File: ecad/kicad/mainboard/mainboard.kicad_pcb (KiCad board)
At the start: 2 copper layers, 99.1 x 81.3 mm, 37 parts, among them IC1 74HC86, J1 SENSORS, J2 CONN_06SILK_FEMALE_PTH, J3 CONN_06SILK_FEMALE_PTH, J4 POWER, J5 SERIAL, M1 Left Motor, M2 Right Motor, U1 Arduino_Nano, U2 TB6612FNG-Module

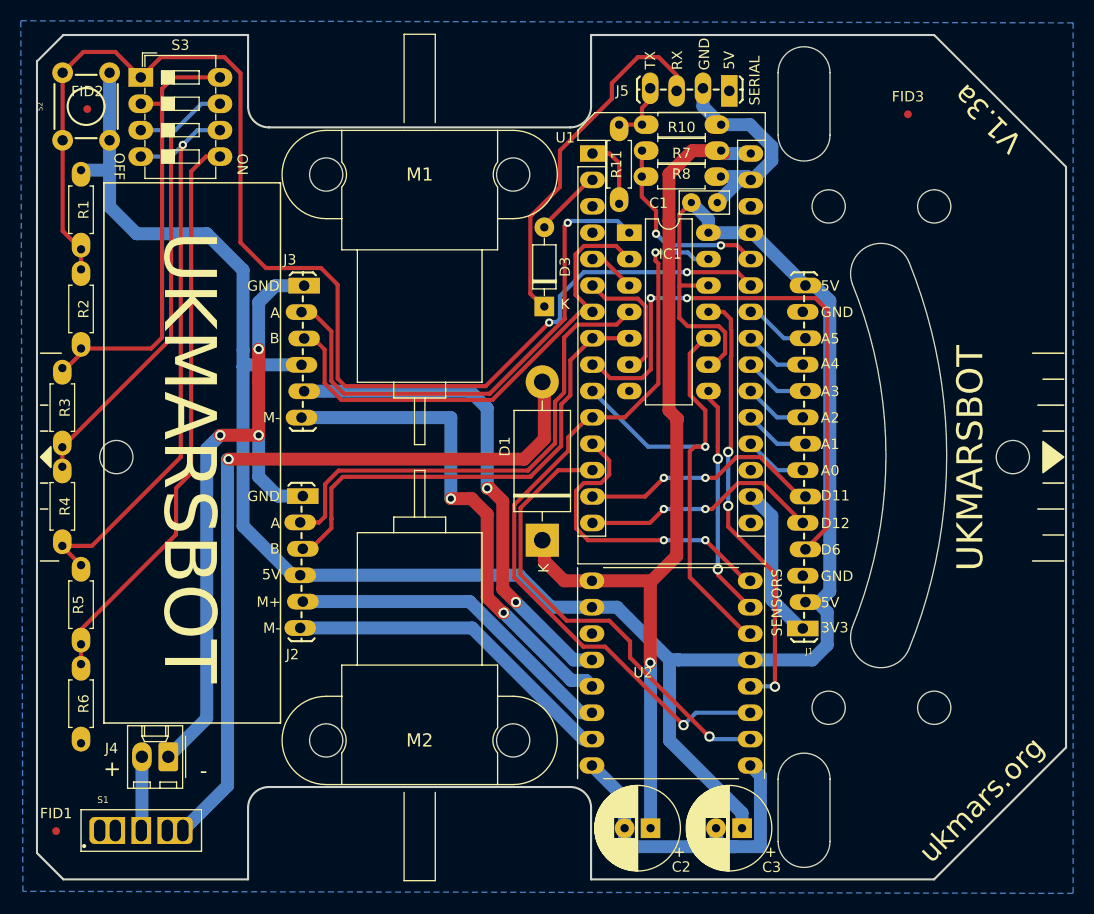
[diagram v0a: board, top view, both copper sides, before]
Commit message: layout
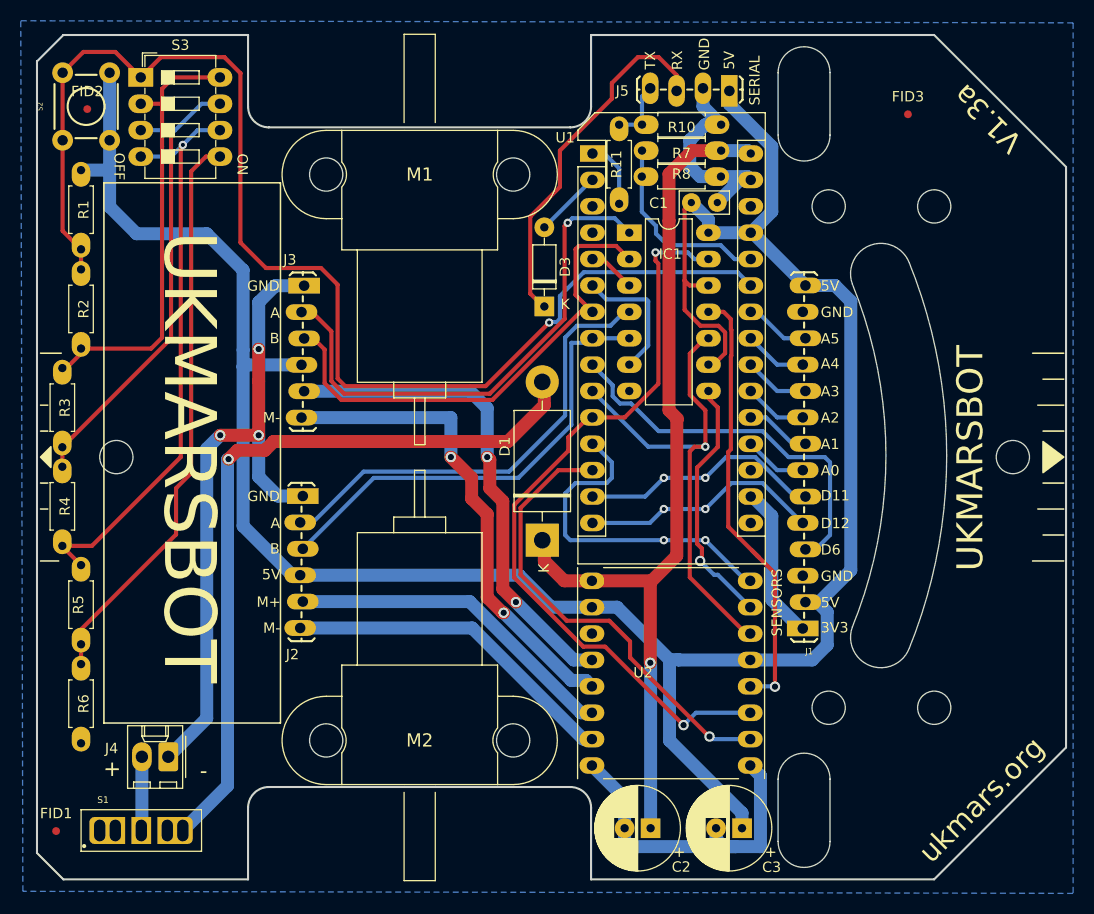
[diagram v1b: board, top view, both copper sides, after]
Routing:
- net 5V: track 220.0 -> 237.5 mm
- net /USER_IO: track 54.3 -> 37.4 mm, vias 2 -> 0
- net /LEFT_PWM: track 29.6 -> 32.9 mm
- net /RIGHT_A: track 47.3 -> 44.5 mm
- net //LEFT_DIR: track 22.8 -> 24.8 mm, vias 2 -> 1
- net /RIGHT_B: track 46.4 -> 44.4 mm
- net unconnected-(S1-Pad1): track 0.00 -> 1.50 mm
- net /LEFT_MOTOR_2: track 47.9 -> 46.8 mm
- net /RIGHT_CLK_A: track 12.7 -> 13.6 mm
- net /EMITTER_A: track 23.1 -> 23.6 mm
- net /V_BATT: track 86.7 -> 86.2 mm
- net //RIGHT_DIR: track 43.4 -> 43.1 mm, vias 3 -> 1
- net /BATTERY_VOLTS: track 18.8 -> 18.7 mm, vias 2 -> 0
- net /FUNCTION_SELECT: vias 2 -> 1
